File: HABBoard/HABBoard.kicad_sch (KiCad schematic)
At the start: 71 parts

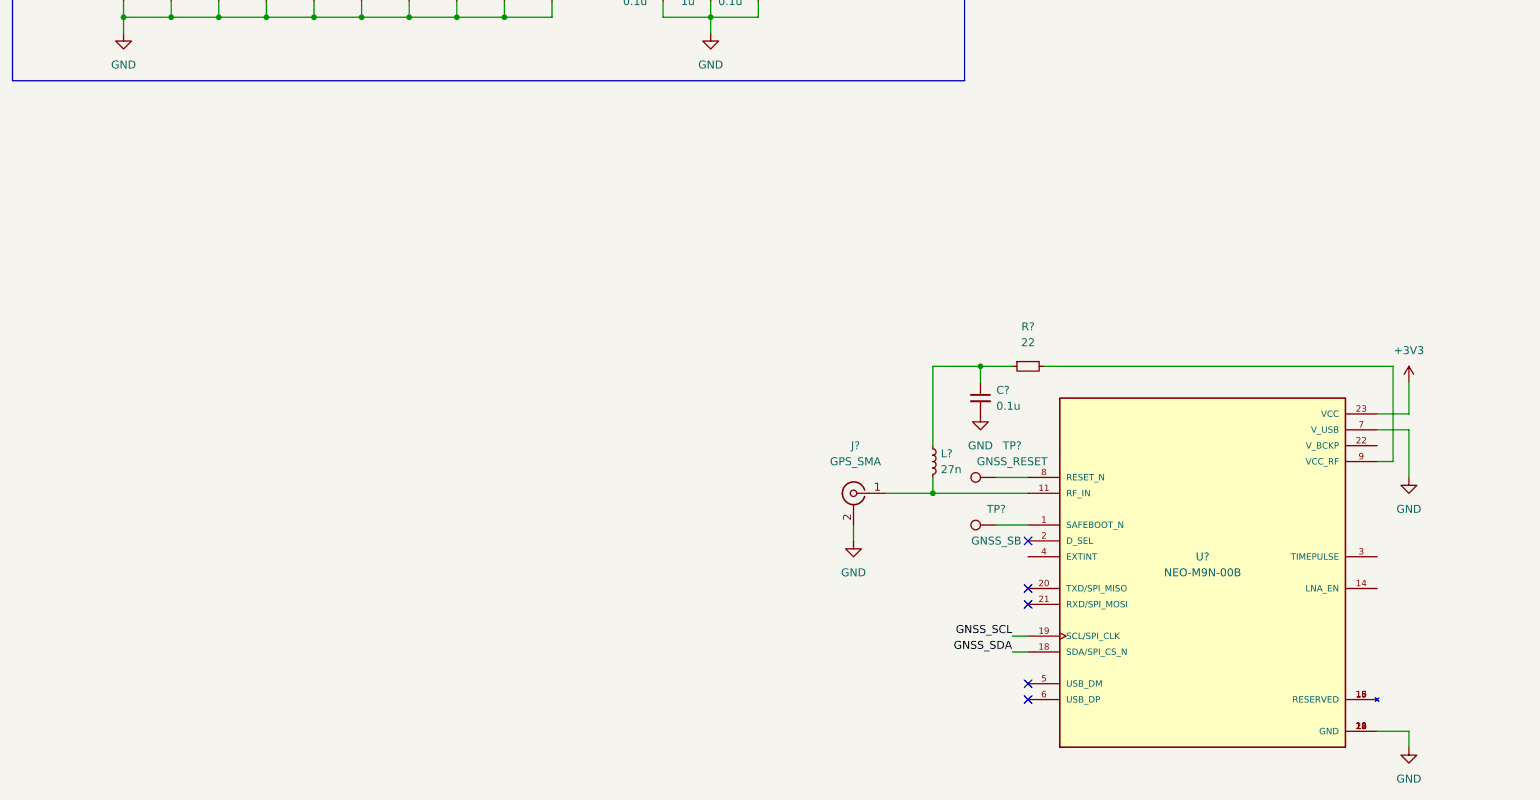
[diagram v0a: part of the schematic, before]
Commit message: Revisions before battery change
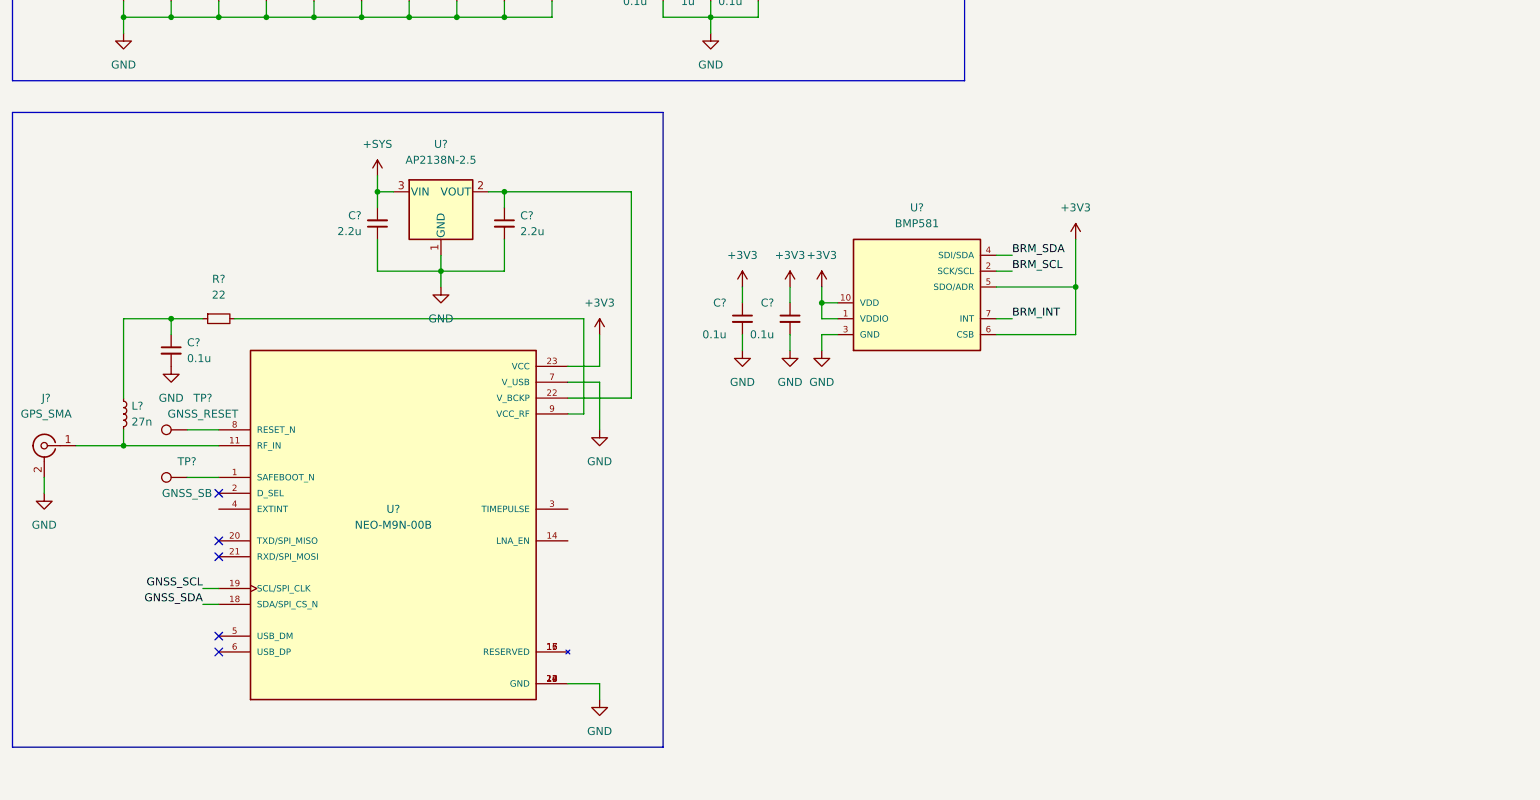
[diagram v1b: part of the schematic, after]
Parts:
- added C? (x2): 0.1u, symbol Device:C_Small
- added C? (x2): 2.2u, symbol Device:C_Small
- added U?: BMP581, HABParts:BMP581, symbol HABParts:BMP581
- added U?: AP2138N-2.5, Package_TO_SOT_SMD:SOT-23, symbol HABParts:AP2138N-2.5
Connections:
- net +3V3: now also C?.1, C?.1, U?.1 (VDDIO), U?.10 (VDD), U?.5 (SDO/ADR), U?.6 (CSB)
- net +SYS: now also C?.2, U?.3 (VIN)
- net GND: now also C?.1, C?.2, C?.2, C?.2, U?.1 (GND), U?.3 (GND), U?.8 (GND), U?.9 (GND)
- net at U?.22 (V_BCKP): now also C?.1, U?.2 (VOUT)
- new net BRM_INT: U?.7 (INT)
- new net BRM_SCL: U?.2 (SCK/SCL)
- new net BRM_SDA: U?.4 (SDI/SDA)
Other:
- moved on the sheet: C?, J?, L?, R?, TP?, U?

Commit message: Added the rest of the sensors
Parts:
- removed BT?: BATT, symbol Device:Battery_Cell
- removed C? (x4): 0.1u, symbol Device:C_Small
- removed C? (x3): 10u, symbol Device:C_Small
- removed C?: 0.47u, symbol Device:C_Small
- removed C? (x3): 2.2u, symbol Device:C_Small
- removed C?: 22u, symbol Device:C_Small
- removed D?: STAT, symbol Device:LED_Small
- removed J?: USB, symbol Connector:USB_C_Receptacle_USB2.0
- removed L?: 0.47u, symbol Device:L_Small
- removed Q? (x2): PMDPB30XN, HABParts:DMN1025UFDB7, symbol HABParts:PMDPB30XN
- removed R?: Rled, symbol Device:R_Small
- removed R?: 100, symbol Device:R_Small
- removed R?: 22, symbol Device:R_Small
- removed R?: 200K, symbol Device:R_Small
- removed R?: Rthm, symbol Device:R_Small
- removed R?: 1K, symbol Device:R_Small
- removed R?: 18.7K, symbol Device:R_Small
- removed R?: 10m, symbol Device:R_Small
- removed R?: 2.26m, symbol Device:R_Small
- removed TH?: THM, symbol Device:Thermistor_NTC
- removed TP?: GNSS_RESET, symbol Connector:TestPoint
- removed U?: TC7USB40FT, Package_SO:TSSOP-14_4.4x5mm_P0.65mm, symbol HABParts:TC7USB40FT
- removed U?: MAX77757JEFG420+, HABParts:IC_MAX77757JEFG420+, symbol HABParts:MAX77757JEFG420+
- removed U?: bq298215, symbol HABParts:bq298215
- removed U?: MAX17260SETD, Package_DFN_QFN:TDFN-14-1EP_3x3mm_P0.4mm_EP1.78x2.35mm, symbol HABParts:MAX17260SETD
- added C? (x2): 2.2u, symbol Device:C_Small
- added C? (x5): 0.1u, symbol Device:C_Small
- added R? (x2): 2.2K, symbol Device:R_Small
- added R? (x2): 10K (DNF), symbol Device:R_Small
- added SW?: RESET, symbol Switch:SW_Push
- added U?: AP2138N-1.8, Package_TO_SOT_SMD:SOT-23, symbol HABParts:AP2138N-1.8
- added U?: ADT7410TRZ, SOIC127P600X175-8N_ADT7410TRZ, symbol HABParts:ADT7410TRZ
- added U?: Si4063, Package_DFN_QFN:QFN-20-1EP_4x4mm_P0.5mm_EP2.6x2.6mm_ThermalVias, symbol HABParts:Si4063
- added U?: ICM-20948, Sensor_Motion:InvenSense_QFN-24_3x3mm_P0.4mm, symbol Sensor_Motion:ICM-20948
- added U?: TXS0104E, Package_SO:TSSOP-14_4.4x5mm_P0.65mm, symbol HABParts:TXS0104E
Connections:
- net MCU_DN is gone; now on an unnamed net: U?.46 (USB_DM)
- net MCU_DP is gone; now on an unnamed net: U?.47 (USB_DP)
- net +3V3: now also C?.1, C?.1, C?.2, R?.2, R?.2, U?.14 (VCCB), U?.3 (VIN), U?.6 (VDD), U?.8 (VDD), U?.8 (VDD)
- net GND: now also C?.1, C?.2, C?.2, C?.2, C?.2, C?.2, C?.2, SW?.1, U?.1 (GND), U?.18 (GND), U?.18 (GND), U?.20 (GND), U?.21 (GND), U?.3 (A0), U?.4 (A1), U?.7 (GND), U?.7 (GND)
- net at U?.8 (RESET_N): now also SW?.2
- new net: C?.1, U?.10 (REGOUT)
- new net: R?.1, U?.5 (INT)
- new net: R?.1, U?.6 (CT)
- new net: R?.1, U?.2 (A1), U?.24 (SDA/SDI)
- new net: R?.1, U?.23 (SCL/SCLK), U?.3 (A2)
- new net: U?.12 (INT1), U?.4 (A3)
- new net +1V8: C?.1, C?.1, C?.1, R?.2, R?.2, U?.1 (VCCA), U?.13 (VDD), U?.2 (VOUT), U?.22 (~{CS}), U?.8 (OE), U?.8 (VDDIO)
- new net IMU_INT: U?.12 (B3)
- new net IMU_SCL: U?.11 (B2)
- new net IMU_SDA: U?.10 (B1)
- new net TMP_SCL: U?.1 (SCL)
- new net TMP_SDA: U?.2 (SDA)
- no-connect marks 9 -> 11
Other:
- moved on the sheet: C?, J?, L?, R?, SW?, TP?, U?
